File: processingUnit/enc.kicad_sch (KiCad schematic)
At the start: 15 parts, among them J301 Conn_01x04, SW301 ENC RST, U301 STM32F401C_B-C_Ux, Y301 16Mhz

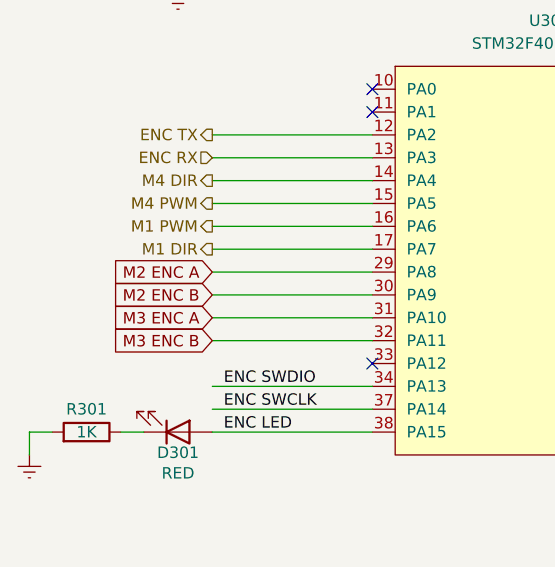
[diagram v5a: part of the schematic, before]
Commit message: schematic
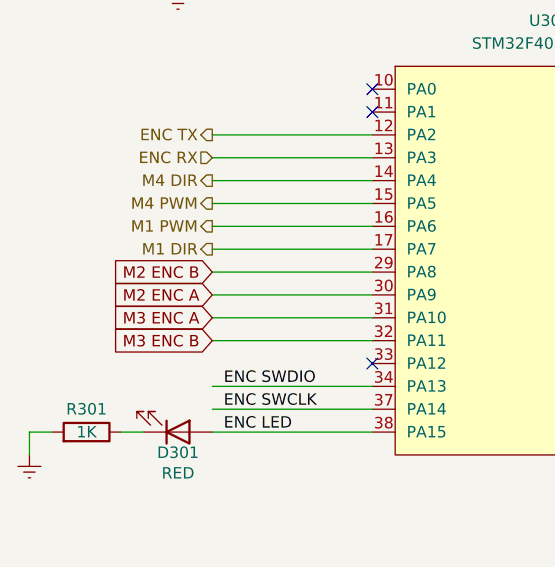
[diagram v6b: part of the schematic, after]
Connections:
- net M2 ENC A: now also U301.30 (PA9); no longer U301.29 (PA8)
- net M2 ENC B: now also U301.29 (PA8); no longer U301.30 (PA9)
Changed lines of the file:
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@@
 	(global_label "M2 ENC A"
 		(shape input)
-		(at 115.57 129.54 180)
+		(at 115.57 132.08 180)
 		(fields_autoplaced yes)
 		(effects
@@
 		)
 		(property "Intersheetrefs" "${INTERSHEET_REFS}"
-			(at 103.1506 129.54 0)
+			(at 102.9692 132.08 0)
 			(effects
 				(font
@@
 	(global_label "M2 ENC B"
 		(shape input)
-		(at 115.57 132.08 180)
+		(at 115.57 129.54 180)
 		(fields_autoplaced yes)
 		(effects
@@
 		)
 		(property "Intersheetrefs" "${INTERSHEET_REFS}"
-			(at 102.9692 132.08 0)
+			(at 103.1506 129.54 0)
 			(effects
 				(font
